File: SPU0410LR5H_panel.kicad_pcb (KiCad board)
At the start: 2 copper layers, 70 x 35 mm, 168 parts, among them J1 Conn_01x04_Pin, U1 MCP6002-xSN, U2 SPU0410LR5H-QB

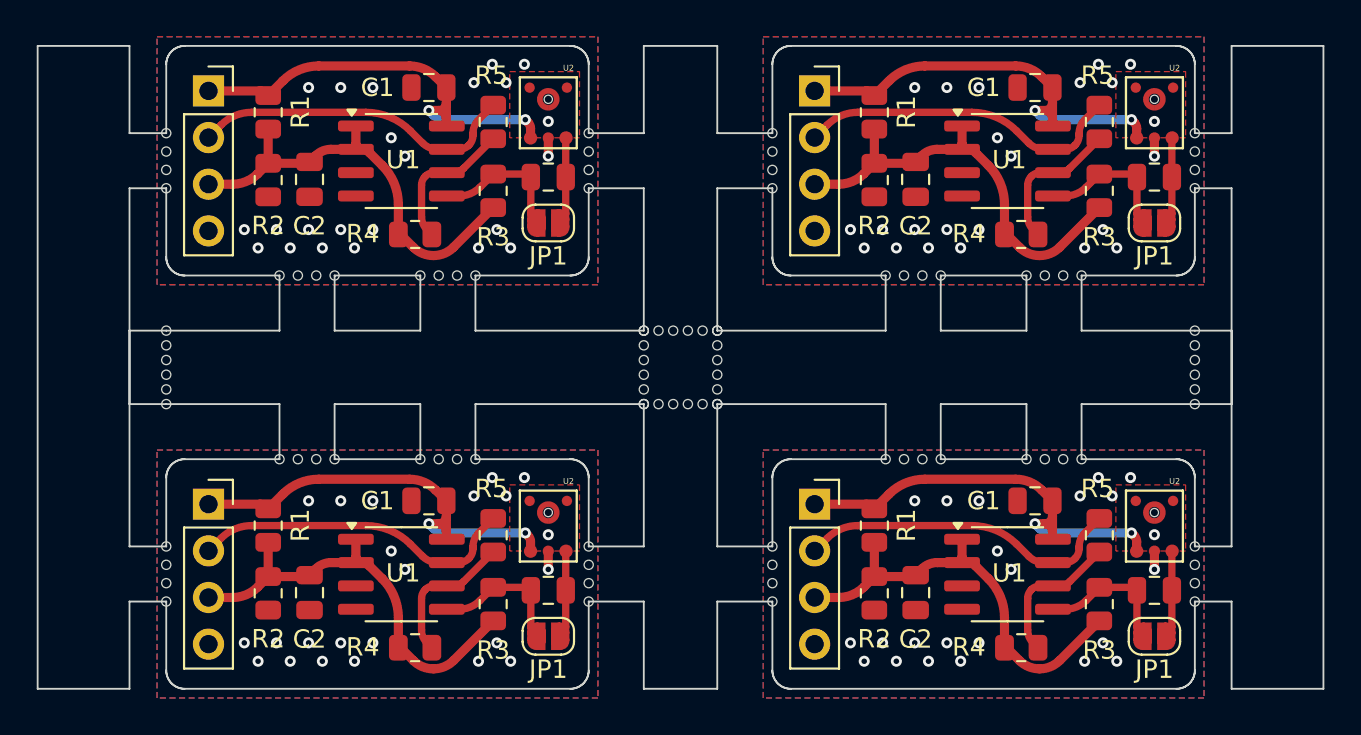
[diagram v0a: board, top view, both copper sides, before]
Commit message: update silkscreen
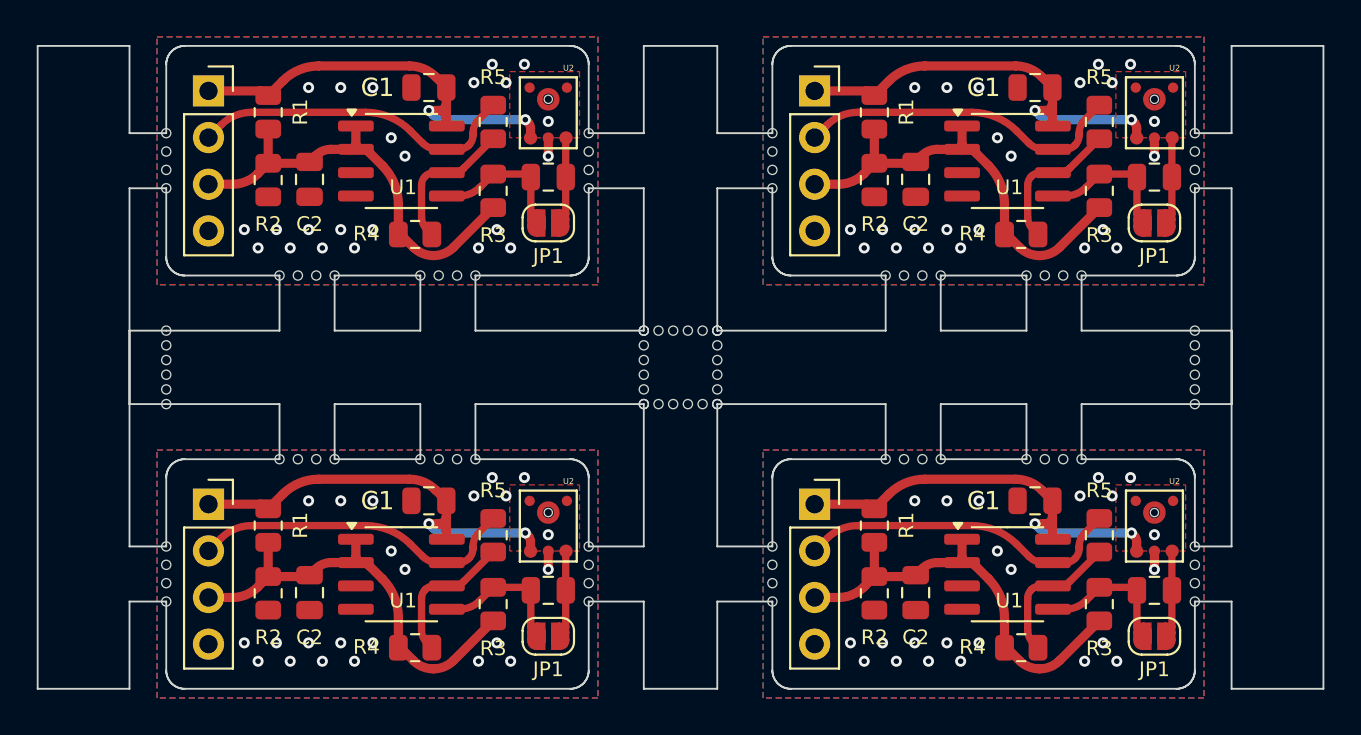
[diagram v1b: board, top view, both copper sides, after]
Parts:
- C3 (x4): value C -> 68n
- R3 (x4): value R -> 100R
- R4 (x4): value R -> 330
- R5 (x4): value R -> 470k
